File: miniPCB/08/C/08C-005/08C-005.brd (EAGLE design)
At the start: 32 parts

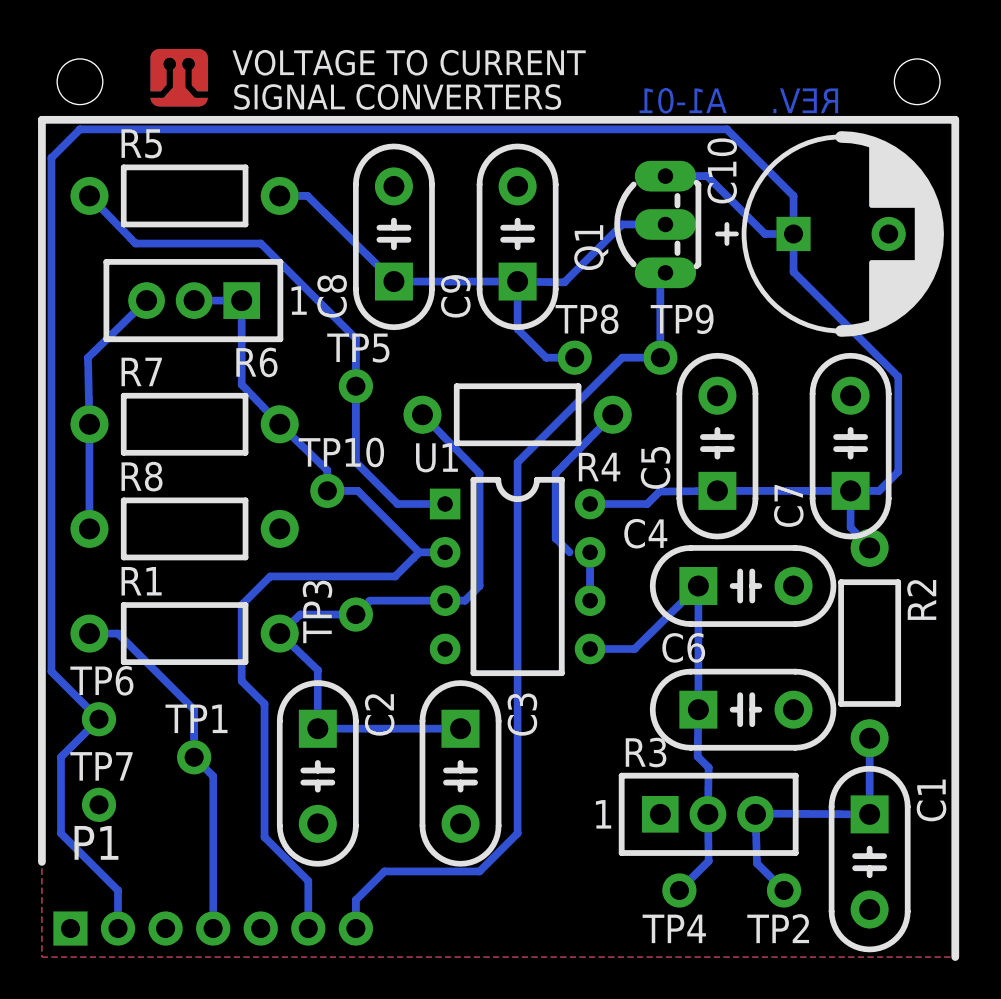
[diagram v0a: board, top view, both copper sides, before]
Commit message: Attempting to fix my Git merge error.
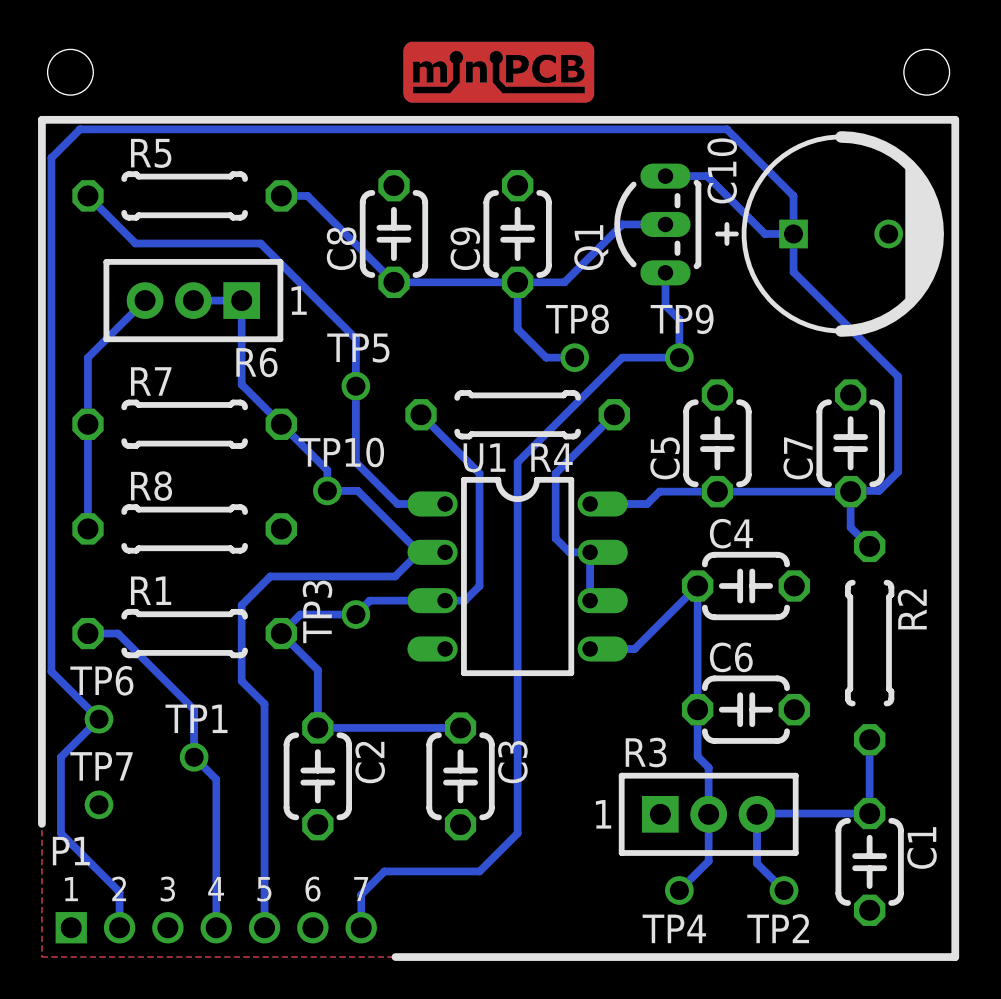
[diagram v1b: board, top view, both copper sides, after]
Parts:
- removed P1: (no value), minipcb:PINS_1X7
- removed PCB1: (no value), minipcb:MINIPCB_0P_50X50MM
- added P1-: (no value), minipcb:MINIPCB_7P_50X50
- moved TP9 1.00 mm to (34.5, 32.5)
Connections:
- net GND: now also P1-.1, P1-.6; no longer P1.1, P1.5
- net N$2: now also P1-.4; no longer P1.4
- net OUT+: now also P1-.7; no longer P1.7
- net OUT-: now also P1-.5; no longer P1.6
- net V+: now also P1-.2; no longer P1.2
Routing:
- net IN: track 11.3 -> 12.4 mm
- net OUT+: track 45.3 -> 46.3 mm
- net OUT-: track 50.8 -> 49.9 mm

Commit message: Attempting to fix my Git merge error.
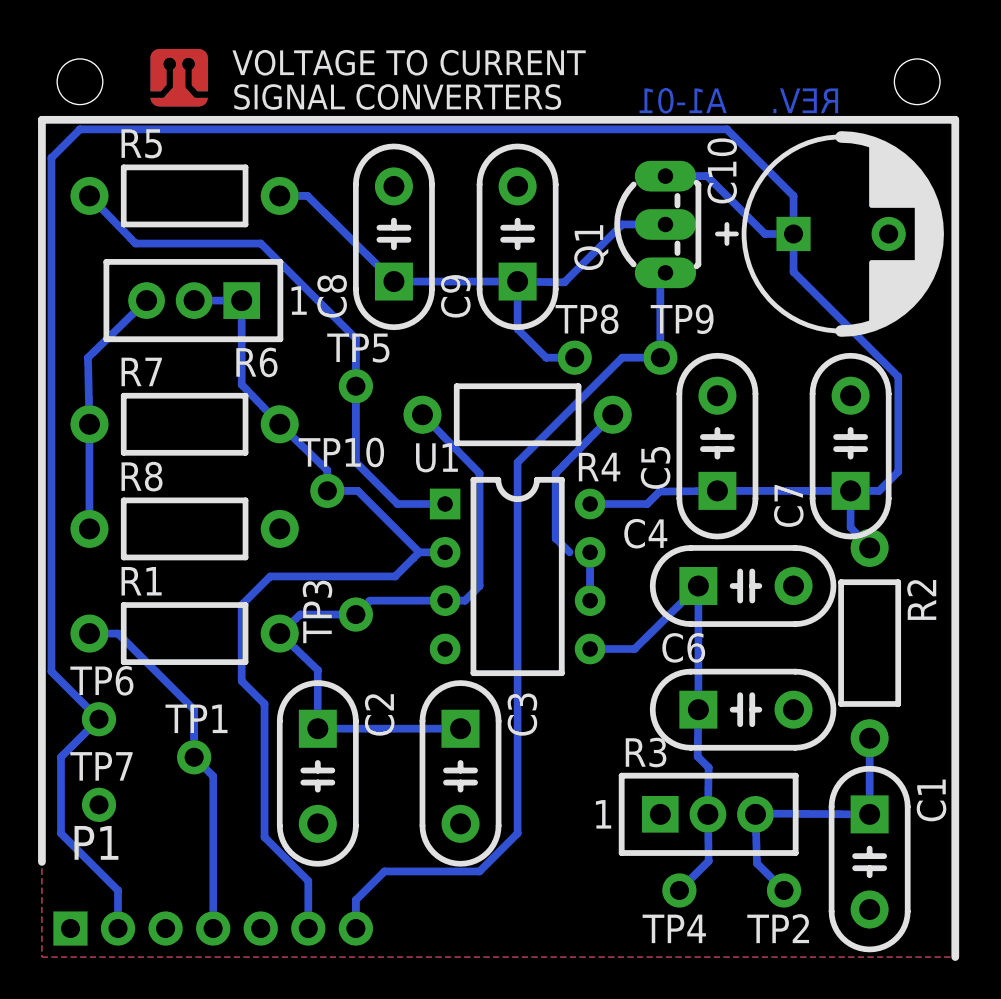
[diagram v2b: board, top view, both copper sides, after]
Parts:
- removed P1-: (no value), minipcb:MINIPCB_7P_50X50
- added P1: (no value), minipcb:PINS_1X7
- added PCB1: (no value), minipcb:MINIPCB_0P_50X50MM
- moved TP9 1.00 mm to (33.5, 32.5)
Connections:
- net GND: now also P1.1, P1.5; no longer P1-.1, P1-.6
- net N$2: now also P1.4; no longer P1-.4
- net OUT+: now also P1.7; no longer P1-.7
- net OUT-: now also P1.6; no longer P1-.5
- net V+: now also P1.2; no longer P1-.2
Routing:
- net IN: track 12.4 -> 11.3 mm
- net OUT+: track 46.3 -> 45.3 mm
- net OUT-: track 49.9 -> 50.8 mm
